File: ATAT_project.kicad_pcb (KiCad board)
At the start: 2 copper layers, 56.2 x 37.9 mm, 32 parts, among them U1 STM32F446RETx, U2 SPBTLE-RF

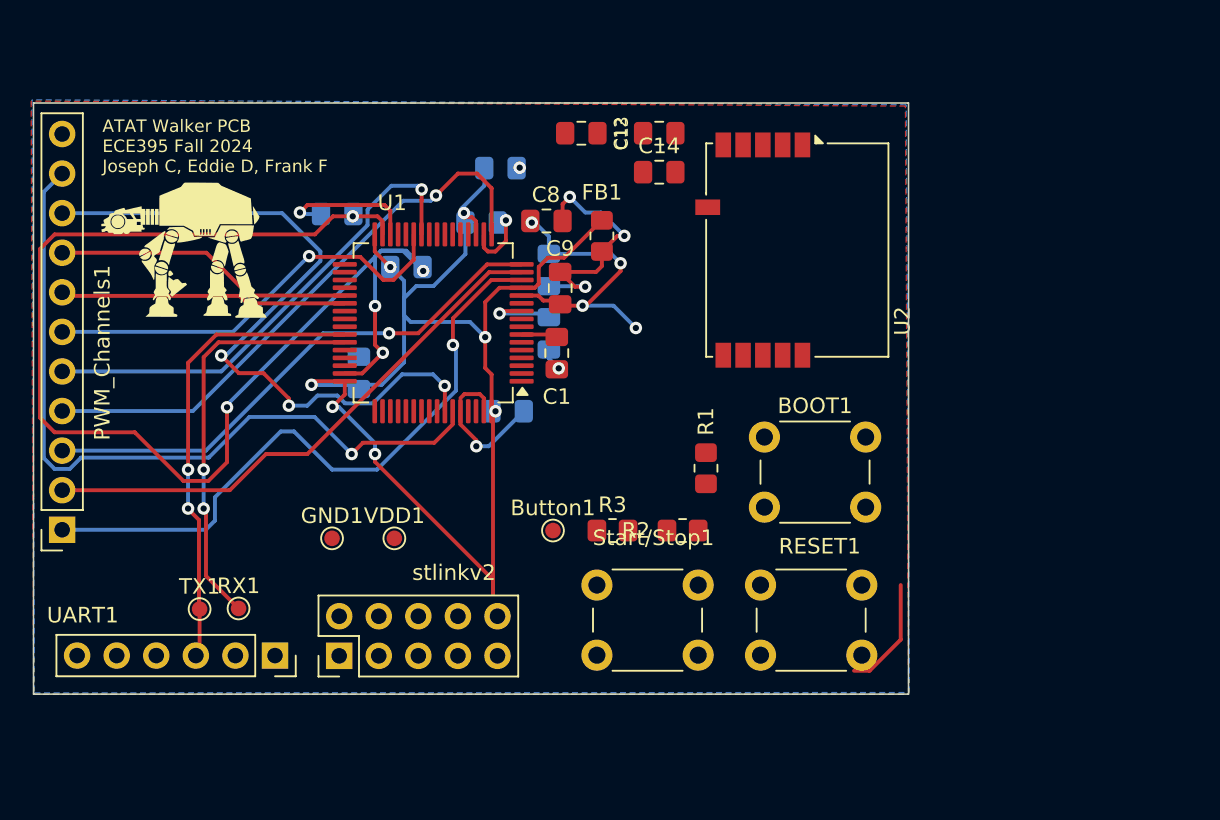
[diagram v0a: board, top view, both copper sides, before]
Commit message: NEW PCB!!!
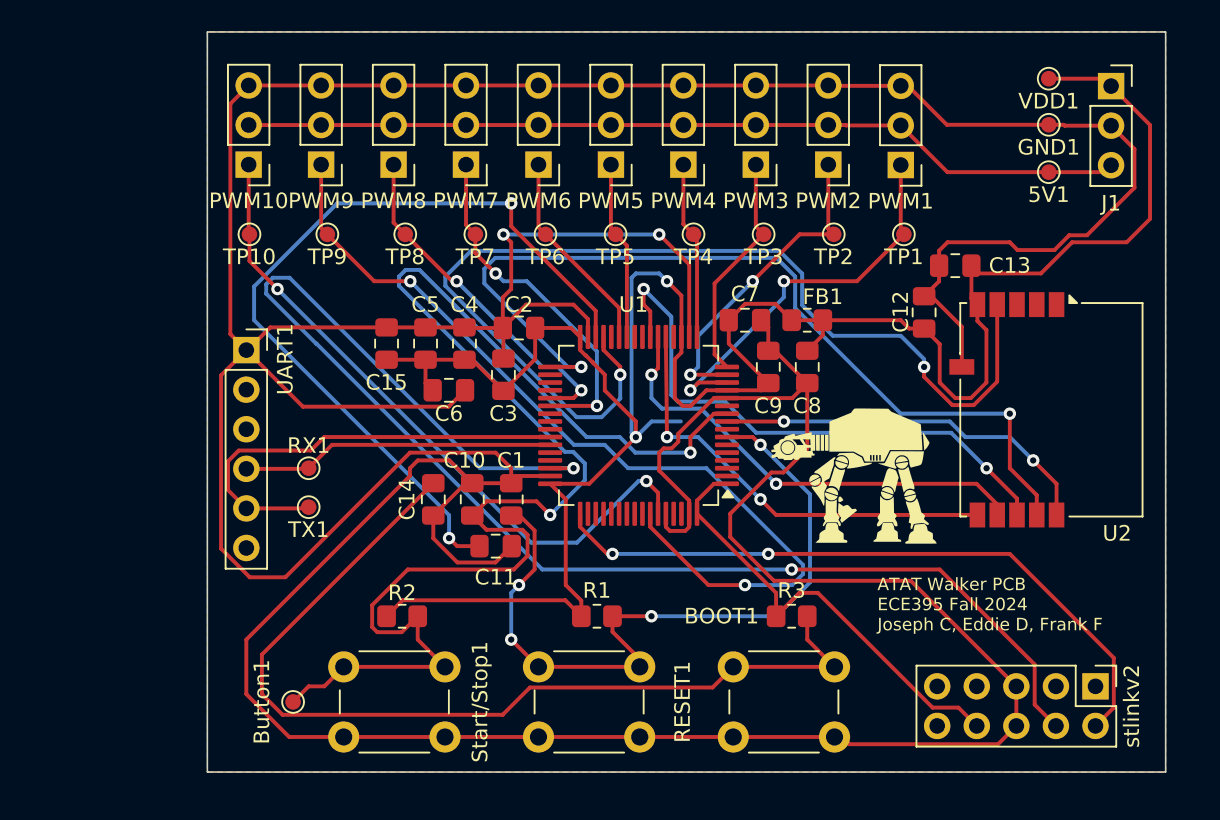
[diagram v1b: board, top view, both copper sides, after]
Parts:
- removed PWM_Channels1: Conn_01x11_Female, Connector_PinSocket_2.54mm:PinSocket_1x11_P2.54mm_Vertical
- added 5V1: Test_5V, TestPoint:TestPoint_Pad_D1.0mm, F.Cu at (151.5, 54.5)
- added C15: 100n, Capacitor_SMD:C_0805_2012Metric_Pad1.18x1.45mm_HandSolder, F.Cu at (109.0, 65.5)
- added J1: Conn_01x03_Socket, Connector_PinSocket_2.54mm:PinSocket_1x03_P2.54mm_Vertical, F.Cu at (155.5, 49.0)
- added PWM1: Conn_01x03_Pin, Connector_PinHeader_2.54mm:PinHeader_1x03_P2.54mm_Vertical, F.Cu at (142.0, 54.0)
- added PWM10: Conn_01x03_Pin, Connector_PinHeader_2.54mm:PinHeader_1x03_P2.54mm_Vertical, F.Cu at (100.2, 54.0)
- added PWM2: Conn_01x03_Pin, Connector_PinHeader_2.54mm:PinHeader_1x03_P2.54mm_Vertical, F.Cu at (137.3, 54.0)
- added PWM3: Conn_01x03_Pin, Connector_PinHeader_2.54mm:PinHeader_1x03_P2.54mm_Vertical, F.Cu at (132.7, 54.0)
- added PWM4: Conn_01x03_Pin, Connector_PinHeader_2.54mm:PinHeader_1x03_P2.54mm_Vertical, F.Cu at (128.1, 54.0)
- added PWM5: Conn_01x03_Pin, Connector_PinHeader_2.54mm:PinHeader_1x03_P2.54mm_Vertical, F.Cu at (123.4, 54.0)
- added PWM6: Conn_01x03_Pin, Connector_PinHeader_2.54mm:PinHeader_1x03_P2.54mm_Vertical, F.Cu at (118.8, 54.0)
- added PWM7: Conn_01x03_Pin, Connector_PinHeader_2.54mm:PinHeader_1x03_P2.54mm_Vertical, F.Cu at (114.1, 54.0)
- added PWM8: Conn_01x03_Pin, Connector_PinHeader_2.54mm:PinHeader_1x03_P2.54mm_Vertical, F.Cu at (109.5, 54.0)
- added PWM9: Conn_01x03_Pin, Connector_PinHeader_2.54mm:PinHeader_1x03_P2.54mm_Vertical, F.Cu at (104.8, 54.0)
- added TP1: Test_PWM, TestPoint:TestPoint_Pad_D1.0mm, F.Cu at (142.2, 58.5)
- added TP10: Test_PWM, TestPoint:TestPoint_Pad_D1.0mm, F.Cu at (100.2, 58.5)
- added TP2: Test_PWM, TestPoint:TestPoint_Pad_D1.0mm, F.Cu at (137.7, 58.5)
- added TP3: Test_PWM, TestPoint:TestPoint_Pad_D1.0mm, F.Cu at (133.2, 58.5)
- added TP4: Test_PWM, TestPoint:TestPoint_Pad_D1.0mm, F.Cu at (128.7, 58.5)
- added TP5: Test_PWM, TestPoint:TestPoint_Pad_D1.0mm, F.Cu at (123.7, 58.5)
- added TP6: Test_PWM, TestPoint:TestPoint_Pad_D1.0mm, F.Cu at (119.2, 58.5)
- added TP7: Test_PWM, TestPoint:TestPoint_Pad_D1.0mm, F.Cu at (114.7, 58.5)
- added TP8: Test_PWM, TestPoint:TestPoint_Pad_D1.0mm, F.Cu at (110.2, 58.5)
- added TP9: Test_PWM, TestPoint:TestPoint_Pad_D1.0mm, F.Cu at (105.2, 58.5)
- C10, C11, C2, C3, C4, C5, C6, C7: moved to F.Cu
- moved GND1 53.1 mm to (151.5, 51.5), turned to 180 degrees
- moved VDD1 51.3 mm to (151.5, 48.5), turned to 180 degrees
- moved stlinkv2 48.6 mm to (154.5, 87.5), turned to -90 degrees
- moved G*** 45.4 mm to (139.0, 74.0)
- moved C14 25.5 mm to (112.0, 75.5), turned to 90 degrees
- moved C12 24.8 mm to (143.5, 63.5), turned to -90 degrees
- moved C11 23.6 mm to (116.0, 78.5)
- moved C13 20.8 mm to (145.5, 60.5)
- moved Button1 20.0 mm to (103.0, 88.5), turned to 90 degrees
- moved UART1 19.7 mm to (100.0, 65.9), turned to 0 degrees
- moved U2 19.3 mm to (148.8, 69.8)
- moved C8 19.2 mm to (136.0, 67.0), turned to -90 degrees
- moved R2 18.8 mm to (110.0, 83.0), turned to 0 degrees
- moved Start/Stop1 17.1 mm to (112.8, 90.8)
- moved RESET1 15.2 mm to (125.2, 90.8)
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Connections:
- net Net-(U1-PA5) renamed SPI_CLK
- net Net-(U1-PA6) renamed SPI_MISO
- net Net-(U1-PA7) renamed SPI_MOSI
- net Net-(U1-PB10) renamed SPI_IRQ
- net Net-(U1-PB12) renamed SPI_CS
- net Net-(U1-PC1) renamed BT_RESET
- C12 pad 2: +3V3 -> +3.3V
- C13 pad 2: +3V3 -> +3.3V
- C2 pad 1: +3V3 -> +3.3V
- C3 pad 1: +3V3 -> +3.3V
- C4 pad 1: +3V3 -> +3.3V
- C5 pad 1: +3V3 -> +3.3V
- C6 pad 1: +3V3 -> +3.3V
- C7 pad 1: +3V3 -> +3.3V
- C8 pad 1: +3V3 -> +3.3V
- C9 pad 1: +3V3 -> +3.3V
- FB1 pad 1: +3V3 -> +3.3V
- FB1 pad 2: +3V3 -> +3.3V
- RX1 pad 1: /RX -> /MCU_RX
- TX1 pad 1: /TX -> /MCU_TX
- U1 pad 1: +3V3 -> +3.3V
- U1 pad 13: +3V3 -> +3.3V
- U1 pad 14: Net-(PWM_Channels1-Pin_1) -> PWM1
- U1 pad 15: Net-(PWM_Channels1-Pin_2) -> PWM2
- U1 pad 16: Net-(PWM_Channels1-Pin_3) -> PWM3
- U1 pad 17: Net-(PWM_Channels1-Pin_4) -> PWM4
- U1 pad 19: +3V3 -> +3.3V
- U1 pad 26: Net-(PWM_Channels1-Pin_5) -> PWM5
- U1 pad 27: Net-(PWM_Channels1-Pin_6) -> PWM6
- U1 pad 32: +3V3 -> +3.3V
- U1 pad 37: Net-(PWM_Channels1-Pin_8) -> PWM8
- U1 pad 38: Net-(PWM_Channels1-Pin_7) -> PWM7
- U1 pad 42: /TX -> /MCU_TX
- U1 pad 43: /RX -> /MCU_RX
- U1 pad 48: +3V3 -> +3.3V
- U1 pad 58: Net-(PWM_Channels1-Pin_9) -> PWM9
- U1 pad 59: Net-(PWM_Channels1-Pin_10) -> PWM10
- U1 pad 64: +3V3 -> +3.3V
- U2 pad 5: +3V3 -> +3.3V
- UART1 pad 1: unconnected-(UART1-Pin_1-Pad1) -> GND
- UART1 pad 2: /RX -> unconnected-(UART1-Pin_2-Pad2)
- UART1 pad 3: /TX -> unconnected-(UART1-Pin_3-Pad3)
- UART1 pad 4: unconnected-(UART1-Pin_4-Pad4) -> /MCU_RX
- UART1 pad 5: unconnected-(UART1-Pin_5-Pad5) -> /MCU_TX
- UART1 pad 6: GND -> unconnected-(UART1-Pin_6-Pad6)
- VDD1 pad 1: +3V3 -> +3.3V
- stlinkv2 pad 8: +3V3 -> +3.3V
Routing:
- net GND: track 124.9 -> 360.3 mm, vias 13 -> 2
- net +3.3V: track 0.00 -> 178.8 mm, vias 0 -> 2
- net +3V3: track 106.3 -> 0.00 mm, vias 10 -> 0
- net /swdio: track 0.00 -> 90.8 mm, vias 0 -> 2
- net Net-(U1-PC2): track 4.75 -> 91.2 mm, vias 1 -> 2
- net SPI_IRQ: track 0.00 -> 67.8 mm, vias 0 -> 2
- net Net-(BOOT1-Pad1): track 0.00 -> 60.6 mm
- net SPI_CS: track 0.00 -> 57.9 mm, vias 0 -> 2
- net PWM9: track 0.00 -> 57.0 mm, vias 0 -> 2
- net +5V: track 0.00 -> 56.8 mm
- net Net-(PWM_Channels1-Pin_10): track 49.3 -> 0.00 mm, vias 1 -> 0
- net Net-(U1-NRST): track 2.32 -> 48.5 mm, vias 0 -> 4
- net Net-(PWM_Channels1-Pin_9): track 46.2 -> 0.00 mm, vias 3 -> 0
- net Net-(U1-VCAP_1): track 9.06 -> 53.0 mm, vias 1 -> 2
- net /swclk: track 0.00 -> 43.4 mm, vias 0 -> 2
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- added copper zone on F.Cu, net (none)
- added copper zone on B.Cu, net +3.3V
- removed copper zone on B.Cu, net GND
- removed copper zone on F.Cu, net GND
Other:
- board size 56.2 x 37.9 mm -> 61.5 x 47.5 mm
